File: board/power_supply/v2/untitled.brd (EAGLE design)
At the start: 25.1 x 51.4 mm, 20 parts, among them IC1 317EMP, Q1 FDD4141TO252

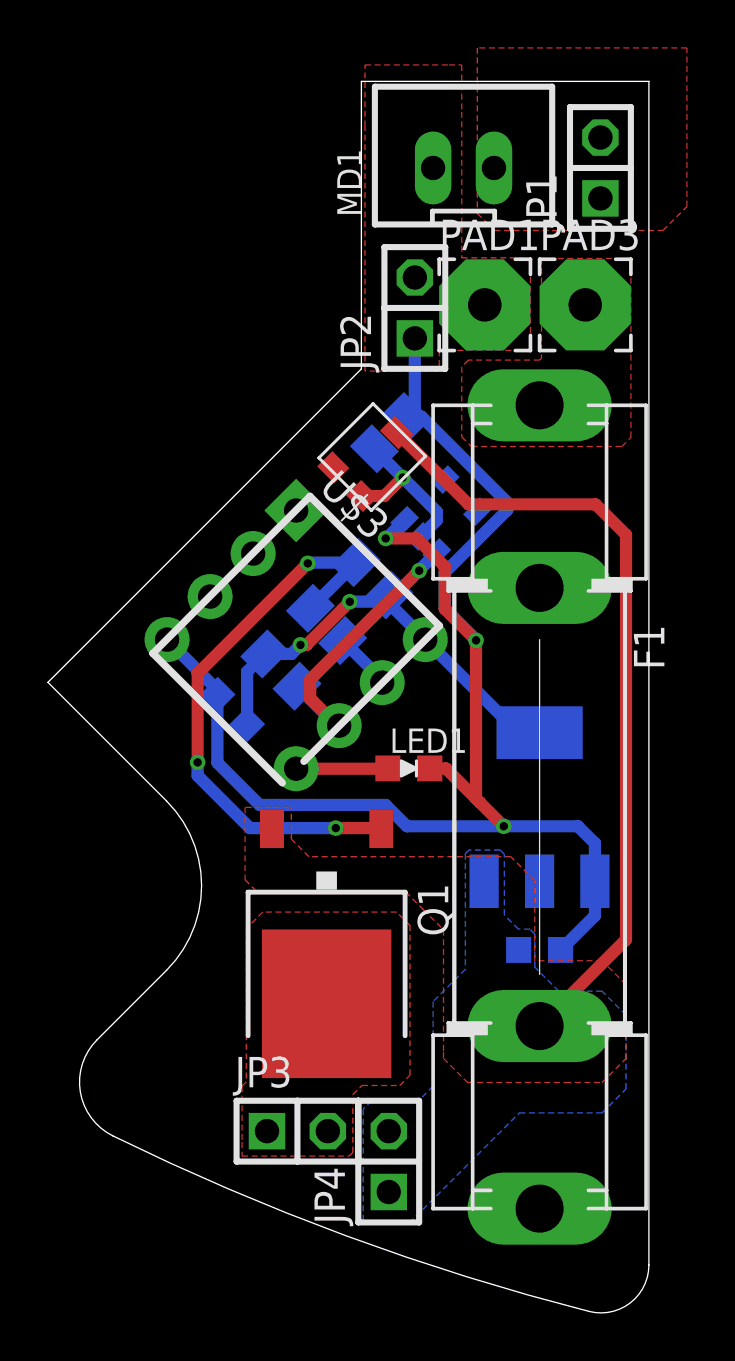
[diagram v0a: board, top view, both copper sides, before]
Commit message: marge前のファイル
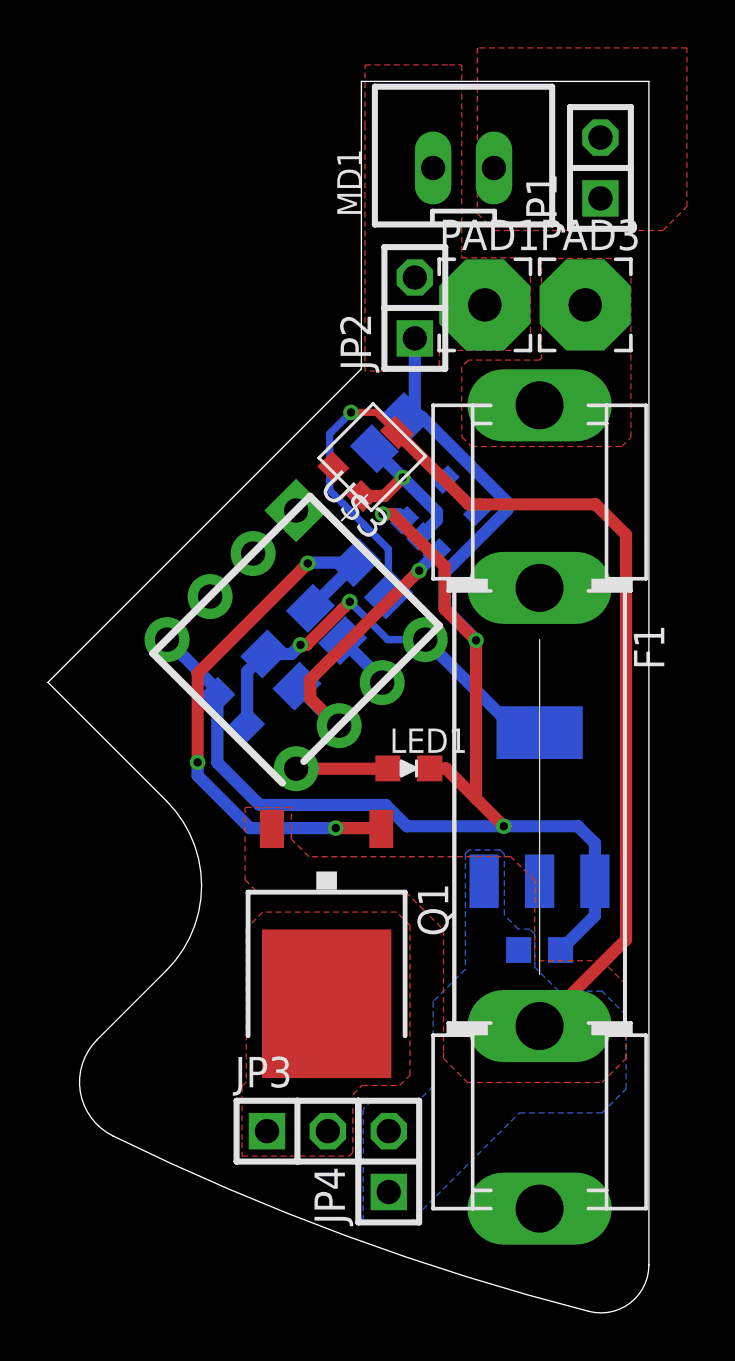
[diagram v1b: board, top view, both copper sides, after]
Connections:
- net N$11: no longer R5.1
- net VCC: now also R5.1
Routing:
- net VCC: track 33.3 -> 44.6 mm, vias 0 -> 1
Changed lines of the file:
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@@
 <?xml version="1.0" encoding="utf-8"?>
 <!DOCTYPE eagle SYSTEM "eagle.dtd">
-<eagle version="9.6.2">
+<eagle version="9.6.1">
 <drawing>
 <settings>
@@
 </layers>
 <board>
-<fusionsync huburn="a.cGVyc29uYWw6dWUyYjhiNWJj" projecturn="a.cGVyc29uYWw6dWUyYjhiNWJjIzIwMjIwNDE2NTE3MzEzNjU2" f3durn="urn:adsk.wipprod:dm.lineage:YKynwMgpTfuc3o3DEV7zsg" pcbguid="" lastpulledtime="" lastsyncedchangeguid="" latestrevisionid="62647a80-3215-48a6-98c3-7560700ce938" lastsyncedrevisionid="62647a80-3215-48a6-98c3-7560700ce938" lastboardhashguid="fa2de31a-8e13-641e-9703-410382d00077" lastpushedtime="2022-10-03T23:37:55Z" linktopcb3d="true"/>
+<fusionsync huburn="a.cGVyc29uYWw6dWUyYjhiNWJj" projecturn="a.cGVyc29uYWw6dWUyYjhiNWJjIzIwMjIwNDE2NTE3MzEzNjU2" f3durn="urn:adsk.wipprod:dm.lineage:YKynwMgpTfuc3o3DEV7zsg" pcbguid="" lastpulledtime="" lastsyncedchangeguid="" latestrevisionid="62647a80-3215-48a6-98c3-7560700ce938" lastsyncedrevisionid="62647a80-3215-48a6-98c3-7560700ce938" lastboardhashguid="fa2de31a-8e13-641e-9703-410382d00077" lastpushedtime="2022-10-03T23:37:55Z" linktopcb3d="%12"/>
 <plain>
 <wire x1="25.083259375" y1="51.943359375" x2="25.083259375" y2="2.542159375" width="0.001" layer="20"/>
@@
 <wire x1="22.1234" y1="20.8534" x2="19.0246" y2="20.8534" width="0.508" layer="16"/>
 <via x="19.0246" y="20.8534" extent="1-16" drill="0.35"/>
-<wire x1="19.0246" y1="20.8534" x2="18.034" y2="21.844" width="0.508" layer="1"/>
-<wire x1="18.034" y1="21.844" x2="17.8689" y2="22.0091" width="0.508" layer="1"/>
+<wire x1="19.0246" y1="20.8534" x2="17.8689" y2="22.0091" width="0.508" layer="1"/>
 <wire x1="22.832440625" y1="20.144359375" x2="22.1234" y2="20.8534" width="0.508" layer="16"/>
 <wire x1="17.8689" y1="22.0091" x2="17.8689" y2="28.6131" width="0.508" layer="1"/>
@@
 <wire x1="8.8392" y1="21.7424" x2="14.097" y2="21.7424" width="0.508" layer="16"/>
 <wire x1="14.097" y1="21.7424" x2="14.986" y2="20.8534" width="0.508" layer="16"/>
-<wire x1="14.8859625" y1="33.623621875" x2="14.129940625" y2="32.8676" width="0.508" layer="16"/>
-<wire x1="14.129940625" y1="32.8676" x2="14.097" y2="32.8676" width="0.508" layer="16"/>
-<via x="14.097" y="32.8676" extent="1-16" drill="0.35"/>
-<wire x1="14.097" y1="32.8676" x2="15.3924" y2="32.8676" width="0.508" layer="1"/>
+<wire x1="14.8859625" y1="33.623621875" x2="14.625984375" y2="33.8836" width="0.508" layer="16"/>
+<wire x1="14.625984375" y1="33.8836" x2="13.97" y2="33.8836" width="0.508" layer="16"/>
+<via x="13.97" y="33.8836" extent="1-16" drill="0.35"/>
+<wire x1="13.97" y1="33.8836" x2="14.3764" y2="33.8836" width="0.508" layer="1"/>
 <wire x1="16.5608" y1="29.9212" x2="17.8689" y2="28.6131" width="0.508" layer="1"/>
-<wire x1="15.3924" y1="32.8676" x2="16.5608" y2="31.6992" width="0.508" layer="1"/>
+<wire x1="14.3764" y1="33.8836" x2="16.5608" y2="31.6992" width="0.508" layer="1"/>
 <wire x1="16.5608" y1="31.6992" x2="16.5608" y2="29.9212" width="0.508" layer="1"/>
 <contactref element="LED1" pad="K"/>
@@
 <wire x1="17.560846875" y1="34.29" x2="22.86" y2="34.29" width="0.508" layer="1"/>
 <wire x1="24.13" y1="33.02" x2="24.13" y2="16.124159375" width="0.508" layer="1"/>
+<contactref element="R5" pad="1"/>
+<wire x1="14.20779375" y1="30.512446875" x2="14.20779375" y2="32.42660625" width="0.3048" layer="16"/>
+<wire x1="11.7602" y1="37.2364" x2="12.6492" y2="38.1254" width="0.3048" layer="16"/>
+<via x="12.6492" y="38.1254" extent="1-16" drill="0.35"/>
+<wire x1="12.6492" y1="38.1254" x2="13.725446875" y2="38.1254" width="0.3048" layer="1"/>
+<wire x1="13.725446875" y1="38.1254" x2="14.56134375" y2="37.289503125" width="0.3048" layer="1"/>
+<wire x1="14.20779375" y1="32.42660625" x2="11.7602" y2="34.8742" width="0.3048" layer="16"/>
+<wire x1="11.7602" y1="34.8742" x2="11.7602" y2="37.2364" width="0.3048" layer="16"/>
 </signal>
 <signal name="N$1">
@@
 <contactref element="C4" pad="2"/>
 <contactref element="U$3" pad="8"/>
-<contactref element="R5" pad="1"/>
 <contactref element="R2" pad="2"/>
 <wire x1="8.312759375" y1="25.10448125" x2="8.312759375" y2="27.30441875" width="0.508" layer="16"/>
 <wire x1="8.312759375" y1="27.30441875" x2="9.054290625" y2="28.04595" width="0.508" layer="16"/>
-<wire x1="15.74919375" y1="28.6442" x2="14.20779375" y2="30.1856" width="0.508" layer="16"/>
-<wire x1="14.20779375" y1="30.1856" x2="14.20779375" y2="30.512446875" width="0.508" layer="16"/>
 <wire x1="15.74919375" y1="28.6442" x2="19.63519375" y2="24.7582" width="0.508" layer="16"/>
 <wire x1="19.63519375" y1="24.7582" x2="20.521040625" y2="24.7582" width="0.508" layer="16"/>
@@
 <wire x1="10.795" y1="28.4226" x2="12.5984" y2="30.226" width="0.508" layer="1"/>
 <via x="12.5984" y="30.226" extent="1-16" drill="0.35"/>
-<wire x1="12.5984" y1="30.226" x2="13.921346875" y2="30.226" width="0.508" layer="16"/>
-<wire x1="13.921346875" y1="30.226" x2="14.20779375" y2="30.512446875" width="0.508" layer="16"/>
+<wire x1="12.5984" y1="30.226" x2="14.1802" y2="28.6442" width="0.3048" layer="16"/>
+<wire x1="14.1802" y1="28.6442" x2="15.74919375" y2="28.6442" width="0.3048" layer="16"/>
 </signal>
 <signal name="N$10">

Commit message: Revert "Merge remote-tracking branch 'origin/Develop' into feature_#37"
This reverts commit cb103155361e8766478c6830db153463370c0739, reversing
changes made to 84e093fe944e1f8653a6822ff34e6f8740617cb5.
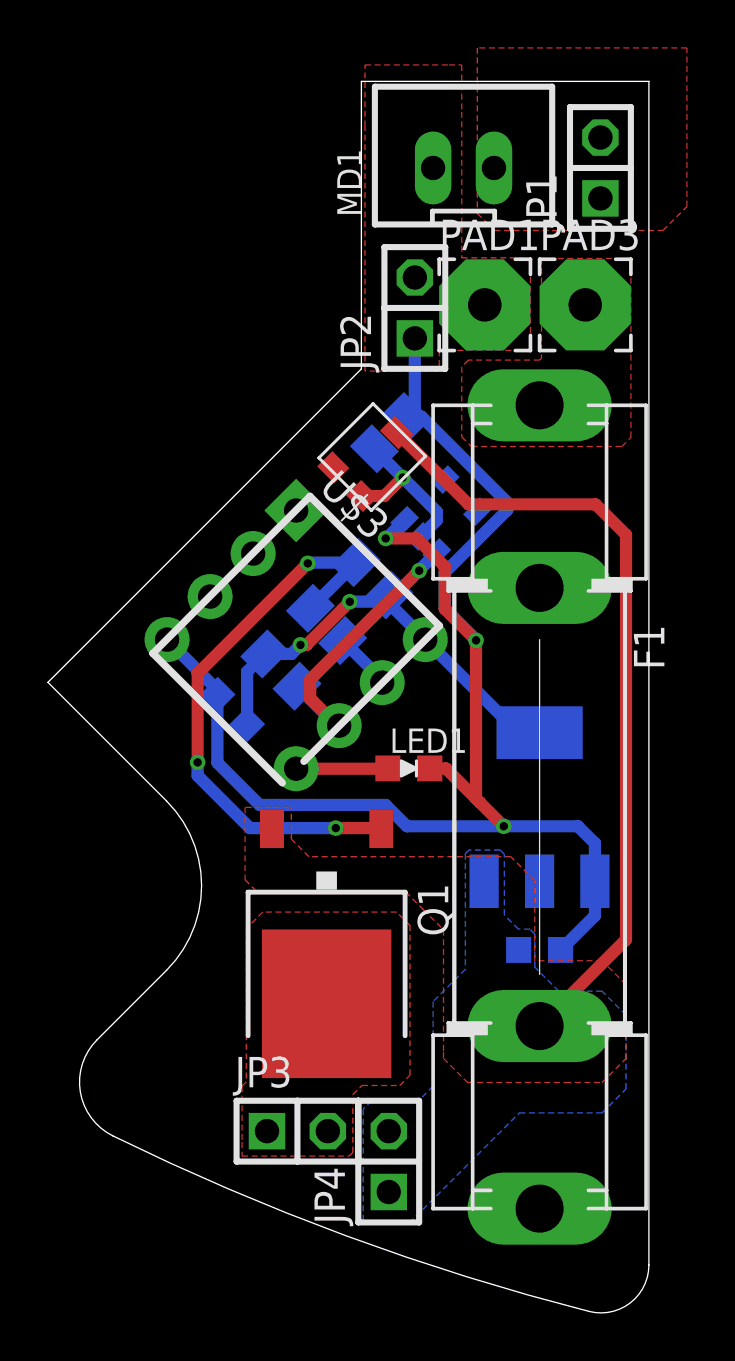
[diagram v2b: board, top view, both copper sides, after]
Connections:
- net N$11: now also R5.1
- net VCC: no longer R5.1
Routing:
- net VCC: track 44.6 -> 33.3 mm, vias 1 -> 0
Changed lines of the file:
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@@
 <?xml version="1.0" encoding="utf-8"?>
 <!DOCTYPE eagle SYSTEM "eagle.dtd">
-<eagle version="9.6.1">
+<eagle version="9.6.2">
 <drawing>
 <settings>
@@
 </layers>
 <board>
-<fusionsync huburn="a.cGVyc29uYWw6dWUyYjhiNWJj" projecturn="a.cGVyc29uYWw6dWUyYjhiNWJjIzIwMjIwNDE2NTE3MzEzNjU2" f3durn="urn:adsk.wipprod:dm.lineage:YKynwMgpTfuc3o3DEV7zsg" pcbguid="" lastpulledtime="" lastsyncedchangeguid="" latestrevisionid="62647a80-3215-48a6-98c3-7560700ce938" lastsyncedrevisionid="62647a80-3215-48a6-98c3-7560700ce938" lastboardhashguid="fa2de31a-8e13-641e-9703-410382d00077" lastpushedtime="2022-10-03T23:37:55Z" linktopcb3d="%12"/>
+<fusionsync huburn="a.cGVyc29uYWw6dWUyYjhiNWJj" projecturn="a.cGVyc29uYWw6dWUyYjhiNWJjIzIwMjIwNDE2NTE3MzEzNjU2" f3durn="urn:adsk.wipprod:dm.lineage:YKynwMgpTfuc3o3DEV7zsg" pcbguid="" lastpulledtime="" lastsyncedchangeguid="" latestrevisionid="62647a80-3215-48a6-98c3-7560700ce938" lastsyncedrevisionid="62647a80-3215-48a6-98c3-7560700ce938" lastboardhashguid="fa2de31a-8e13-641e-9703-410382d00077" lastpushedtime="2022-10-03T23:37:55Z" linktopcb3d="true"/>
 <plain>
 <wire x1="25.083259375" y1="51.943359375" x2="25.083259375" y2="2.542159375" width="0.001" layer="20"/>
@@
 <wire x1="22.1234" y1="20.8534" x2="19.0246" y2="20.8534" width="0.508" layer="16"/>
 <via x="19.0246" y="20.8534" extent="1-16" drill="0.35"/>
-<wire x1="19.0246" y1="20.8534" x2="17.8689" y2="22.0091" width="0.508" layer="1"/>
+<wire x1="19.0246" y1="20.8534" x2="18.034" y2="21.844" width="0.508" layer="1"/>
+<wire x1="18.034" y1="21.844" x2="17.8689" y2="22.0091" width="0.508" layer="1"/>
 <wire x1="22.832440625" y1="20.144359375" x2="22.1234" y2="20.8534" width="0.508" layer="16"/>
 <wire x1="17.8689" y1="22.0091" x2="17.8689" y2="28.6131" width="0.508" layer="1"/>
@@
 <wire x1="8.8392" y1="21.7424" x2="14.097" y2="21.7424" width="0.508" layer="16"/>
 <wire x1="14.097" y1="21.7424" x2="14.986" y2="20.8534" width="0.508" layer="16"/>
-<wire x1="14.8859625" y1="33.623621875" x2="14.625984375" y2="33.8836" width="0.508" layer="16"/>
-<wire x1="14.625984375" y1="33.8836" x2="13.97" y2="33.8836" width="0.508" layer="16"/>
-<via x="13.97" y="33.8836" extent="1-16" drill="0.35"/>
-<wire x1="13.97" y1="33.8836" x2="14.3764" y2="33.8836" width="0.508" layer="1"/>
+<wire x1="14.8859625" y1="33.623621875" x2="14.129940625" y2="32.8676" width="0.508" layer="16"/>
+<wire x1="14.129940625" y1="32.8676" x2="14.097" y2="32.8676" width="0.508" layer="16"/>
+<via x="14.097" y="32.8676" extent="1-16" drill="0.35"/>
+<wire x1="14.097" y1="32.8676" x2="15.3924" y2="32.8676" width="0.508" layer="1"/>
 <wire x1="16.5608" y1="29.9212" x2="17.8689" y2="28.6131" width="0.508" layer="1"/>
-<wire x1="14.3764" y1="33.8836" x2="16.5608" y2="31.6992" width="0.508" layer="1"/>
+<wire x1="15.3924" y1="32.8676" x2="16.5608" y2="31.6992" width="0.508" layer="1"/>
 <wire x1="16.5608" y1="31.6992" x2="16.5608" y2="29.9212" width="0.508" layer="1"/>
 <contactref element="LED1" pad="K"/>
@@
 <wire x1="17.560846875" y1="34.29" x2="22.86" y2="34.29" width="0.508" layer="1"/>
 <wire x1="24.13" y1="33.02" x2="24.13" y2="16.124159375" width="0.508" layer="1"/>
-<contactref element="R5" pad="1"/>
-<wire x1="14.20779375" y1="30.512446875" x2="14.20779375" y2="32.42660625" width="0.3048" layer="16"/>
-<wire x1="11.7602" y1="37.2364" x2="12.6492" y2="38.1254" width="0.3048" layer="16"/>
-<via x="12.6492" y="38.1254" extent="1-16" drill="0.35"/>
-<wire x1="12.6492" y1="38.1254" x2="13.725446875" y2="38.1254" width="0.3048" layer="1"/>
-<wire x1="13.725446875" y1="38.1254" x2="14.56134375" y2="37.289503125" width="0.3048" layer="1"/>
-<wire x1="14.20779375" y1="32.42660625" x2="11.7602" y2="34.8742" width="0.3048" layer="16"/>
-<wire x1="11.7602" y1="34.8742" x2="11.7602" y2="37.2364" width="0.3048" layer="16"/>
 </signal>
 <signal name="N$1">
@@
 <contactref element="C4" pad="2"/>
 <contactref element="U$3" pad="8"/>
+<contactref element="R5" pad="1"/>
 <contactref element="R2" pad="2"/>
 <wire x1="8.312759375" y1="25.10448125" x2="8.312759375" y2="27.30441875" width="0.508" layer="16"/>
 <wire x1="8.312759375" y1="27.30441875" x2="9.054290625" y2="28.04595" width="0.508" layer="16"/>
+<wire x1="15.74919375" y1="28.6442" x2="14.20779375" y2="30.1856" width="0.508" layer="16"/>
+<wire x1="14.20779375" y1="30.1856" x2="14.20779375" y2="30.512446875" width="0.508" layer="16"/>
 <wire x1="15.74919375" y1="28.6442" x2="19.63519375" y2="24.7582" width="0.508" layer="16"/>
 <wire x1="19.63519375" y1="24.7582" x2="20.521040625" y2="24.7582" width="0.508" layer="16"/>
@@
 <wire x1="10.795" y1="28.4226" x2="12.5984" y2="30.226" width="0.508" layer="1"/>
 <via x="12.5984" y="30.226" extent="1-16" drill="0.35"/>
-<wire x1="12.5984" y1="30.226" x2="14.1802" y2="28.6442" width="0.3048" layer="16"/>
-<wire x1="14.1802" y1="28.6442" x2="15.74919375" y2="28.6442" width="0.3048" layer="16"/>
+<wire x1="12.5984" y1="30.226" x2="13.921346875" y2="30.226" width="0.508" layer="16"/>
+<wire x1="13.921346875" y1="30.226" x2="14.20779375" y2="30.512446875" width="0.508" layer="16"/>
 </signal>
 <signal name="N$10">
